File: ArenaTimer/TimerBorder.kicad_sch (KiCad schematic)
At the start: 72 parts

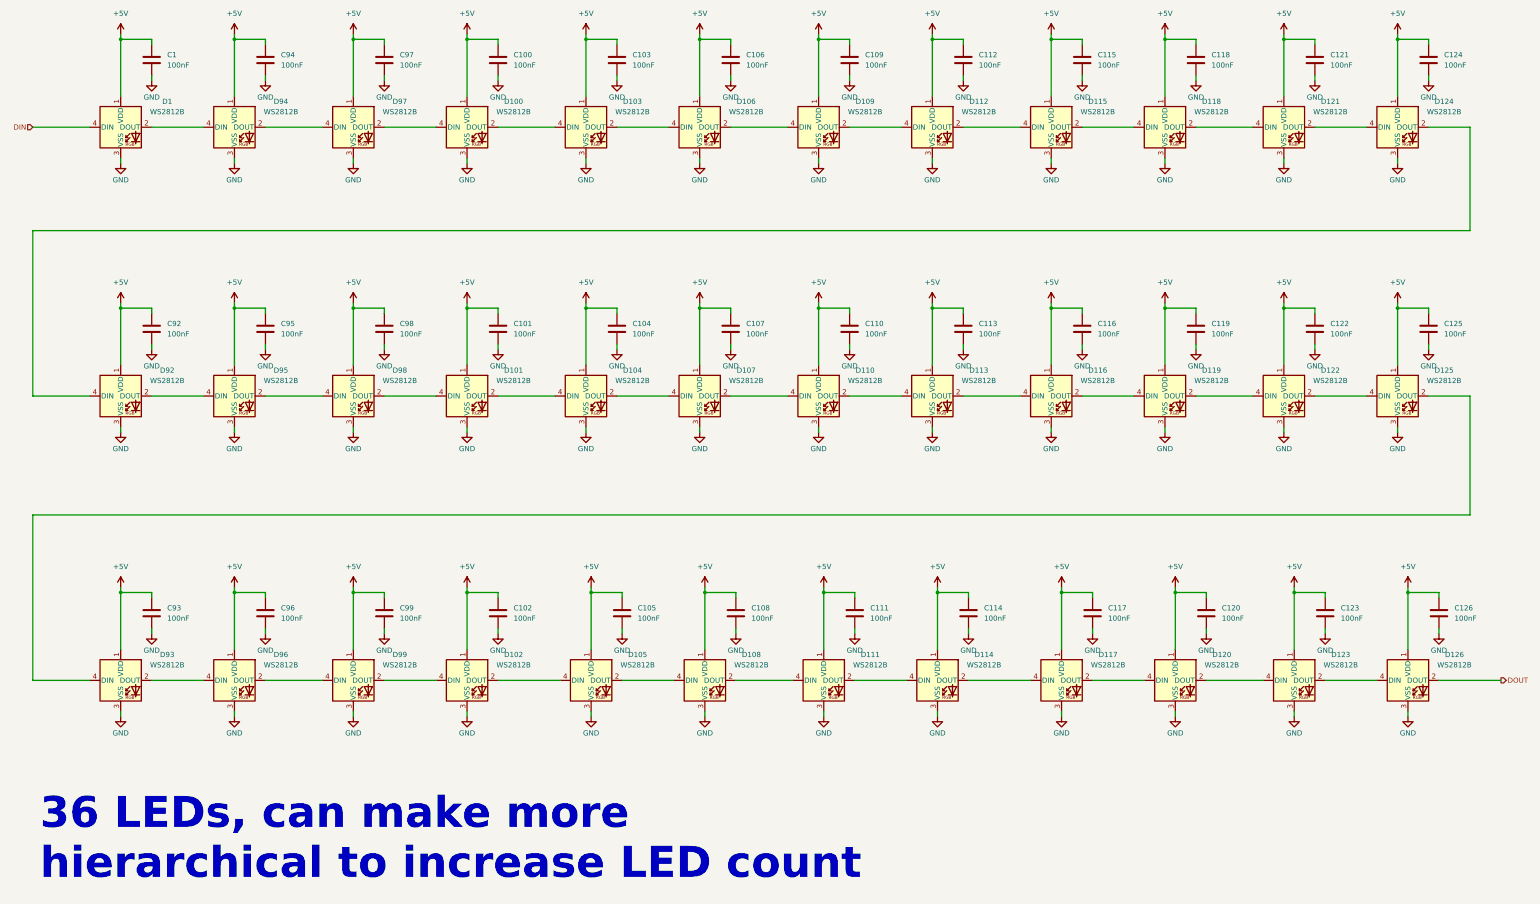
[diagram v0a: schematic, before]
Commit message: finish up routing
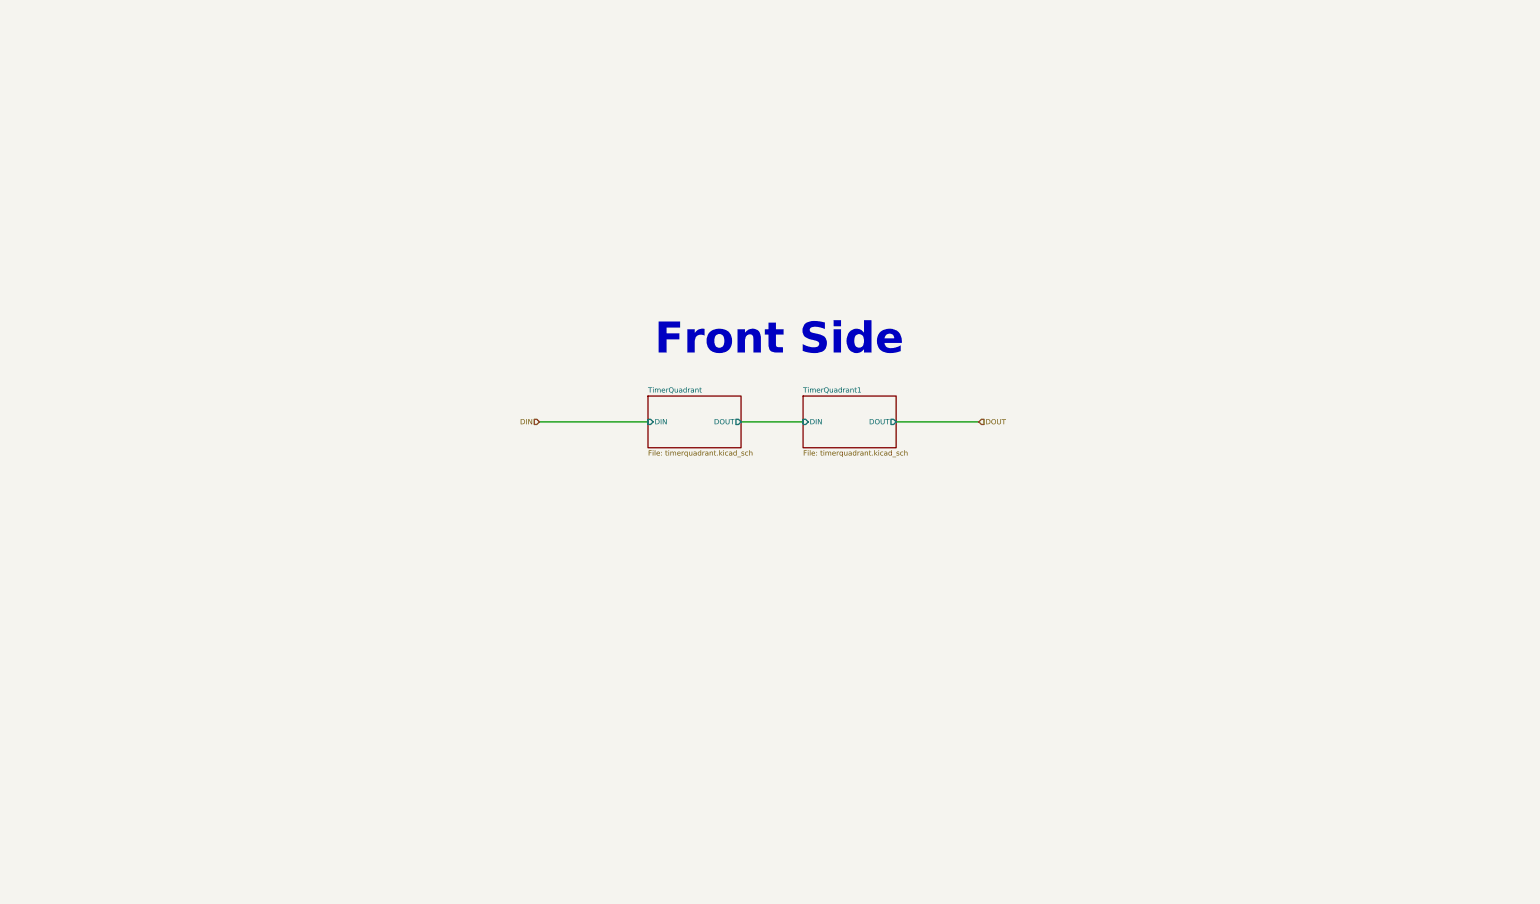
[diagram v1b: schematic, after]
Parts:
- removed C1, C100, C101, C102, C103, C104, C105, C106, C107, C108, C109, C110, C111, C112, C113, C114, C115, C116, C117, C118, C119, C120, C121, C122, C123, C124, C125, C126, C92, C93, C94, C95, C96, C97, C98, C99: 100nF, symbol Device:C
- removed D1, D100, D101, D102, D103, D104, D105, D106, D107, D108, D109, D110, D111, D112, D113, D114, D115, D116, D117, D118, D119, D120, D121, D122, D123, D124, D125, D126, D92, D93, D94, D95, D96, D97, D98, D99: WS2812B, LED_SMD:LED_WS2812B_PLCC4_5.0x5.0mm_P3.2mm, symbol LED:WS2812B
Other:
- added sheet TimerQuadrant (timerquadrant.kicad_sch)
- added sheet TimerQuadrant1 (timerquadrant.kicad_sch)
- note added: "Front Side"
- note removed: "36 LEDs, can make more hierarchical to increase LED count"
